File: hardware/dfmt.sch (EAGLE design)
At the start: 16 parts, among them X1 MINI-USB-32005-201

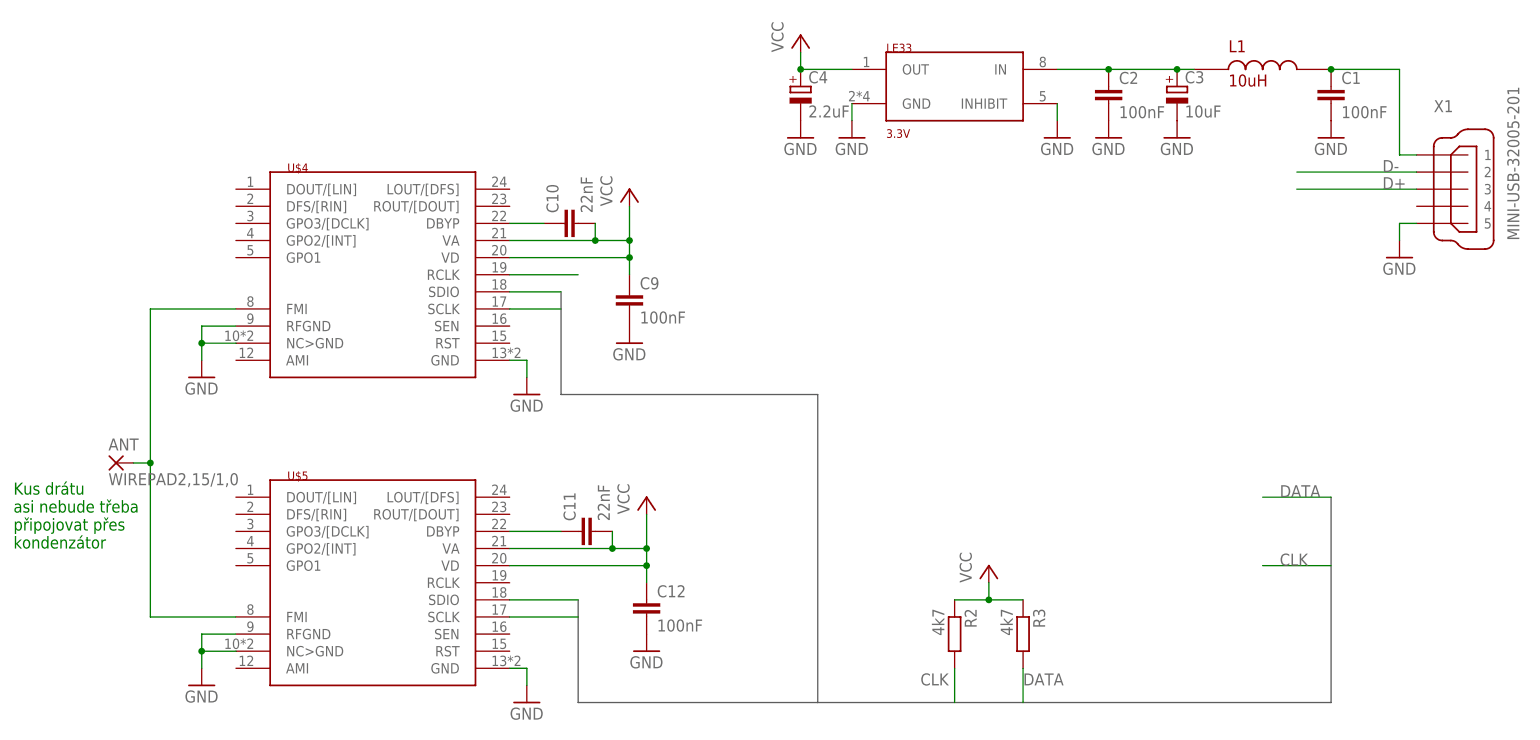
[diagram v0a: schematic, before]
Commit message: working version
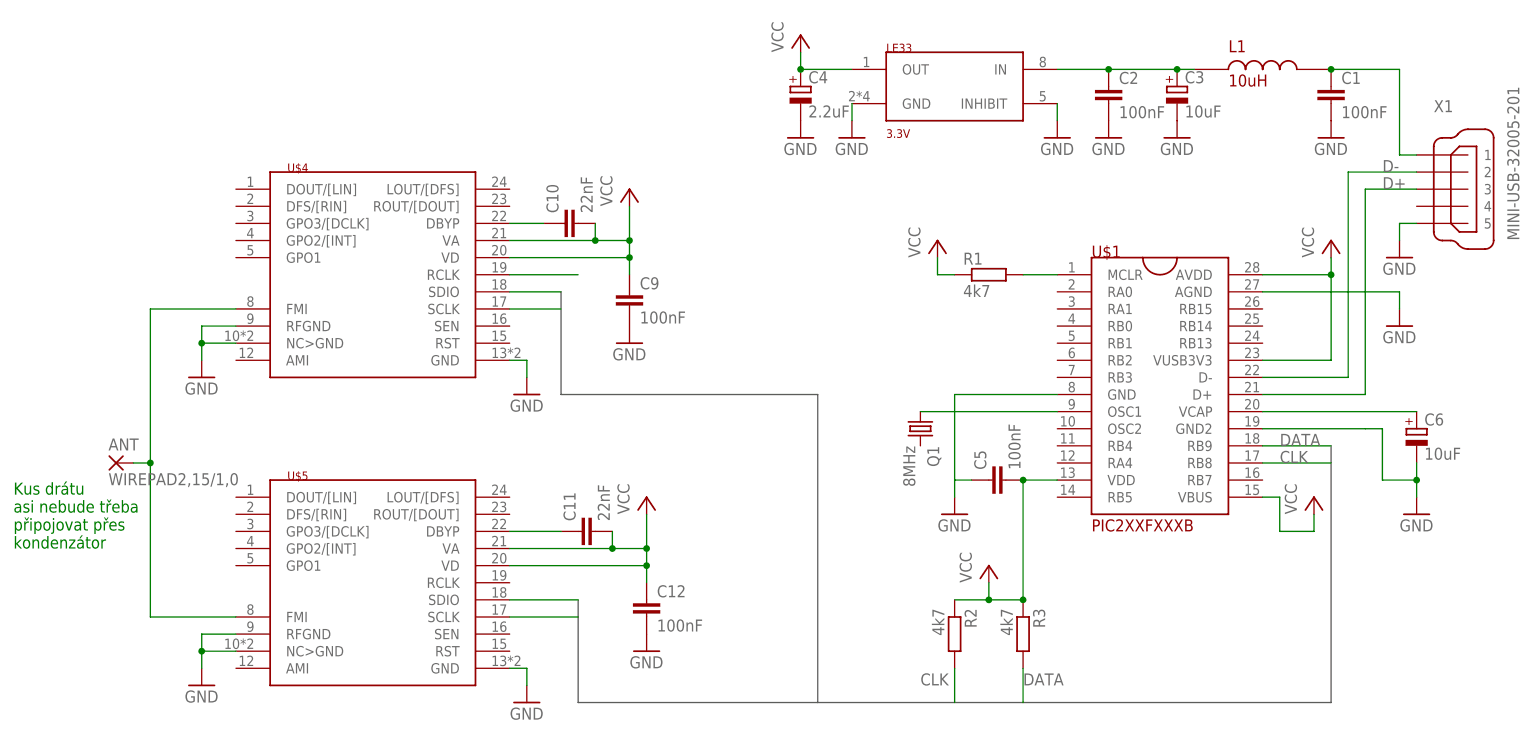
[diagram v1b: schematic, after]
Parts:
- added C5: 100nF, resistor:C-EUC1206
- added C6: 10uF, resistor:CPOL-EUSMCB
- added Q1: 8MHz, crystal:CSM-7X-DU
- added R1: 4k7, resistor:R-EU_R1206
- added U$1: PIC2XXFXXXB, dfmt:PIC2XXFXXXB
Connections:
- new net N$10: U$1.GND2
- new net N$11: Q1.1, U$1.OSC1
- new net N$5: R1.2, U$1.MCLR
- new net N$7: C6.+, U$1.VCAP
- net CLK: now also U$1.RB8
- net D+: now also U$1.D+
- net D-: now also U$1.D-
- net DATA: now also U$1.RB9
- net GND: now also C5.1, C6.-, U$1.AGND, U$1.GND
- net VCC: now also C5.2, R1.1, U$1.AVDD, U$1.VBUS, U$1.VDD, U$1.VUSB3V3
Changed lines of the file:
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@@
 <part name="X1" library="con-cypressindustries" deviceset="MINI-USB-" device="32005-201"/>
 <part name="GND7" library="supply1" deviceset="GND" device=""/>
+<part name="U$1" library="dfmt" deviceset="PIC2XXFXXXB" device=""/>
+<part name="GND8" library="supply1" deviceset="GND" device=""/>
+<part name="GND9" library="supply1" deviceset="GND" device=""/>
+<part name="P+2" library="supply1" deviceset="VCC" device=""/>
+<part name="R1" library="resistor" deviceset="R-EU_" device="R1206" value="4k7"/>
+<part name="P+6" library="supply1" deviceset="VCC" device=""/>
+<part name="C5" library="resistor" deviceset="C-EU" device="C1206" value="100nF"/>
+<part name="C6" library="resistor" deviceset="CPOL-EU" device="SMCB" value="10uF"/>
+<part name="GND16" library="supply1" deviceset="GND" device=""/>
+<part name="P+7" library="supply1" deviceset="VCC" device=""/>
+<part name="Q1" library="crystal" deviceset="CSM-7X-DU" device="" value="8MHz"/>
 </parts>
 <sheets>
@@
 <instance part="X1" gate="G$1" x="58.42" y="50.8"/>
 <instance part="GND7" gate="1" x="50.8" y="40.64"/>
+<instance part="U$1" gate="G$1" x="15.24" y="22.86"/>
+<instance part="GND8" gate="1" x="53.34" y="2.54"/>
+<instance part="GND9" gate="1" x="-15.24" y="2.54"/>
+<instance part="P+2" gate="VCC" x="40.64" y="43.18"/>
+<instance part="R1" gate="G$1" x="-10.16" y="38.1"/>
+<instance part="P+6" gate="VCC" x="-17.78" y="43.18"/>
+<instance part="C5" gate="G$1" x="-10.16" y="7.62" rot="R90"/>
+<instance part="C6" gate="G$1" x="53.34" y="15.24"/>
+<instance part="GND16" gate="1" x="50.8" y="30.48"/>
+<instance part="P+7" gate="VCC" x="38.1" y="5.08"/>
+<instance part="Q1" gate="P" x="-20.32" y="15.24" rot="R270"/>
 </instances>
 <busses>
 <bus name="DATA,CLK">
 <segment>
-<wire x1="40.64" y1="5.08" x2="40.64" y2="-25.4" width="0.762" layer="92"/>
+<wire x1="40.64" y1="12.7" x2="40.64" y2="-25.4" width="0.762" layer="92"/>
 <wire x1="40.64" y1="-25.4" x2="-35.56" y2="-25.4" width="0.762" layer="92"/>
 <wire x1="-35.56" y1="-25.4" x2="-71.12" y2="-25.4" width="0.762" layer="92"/>
@@
 <pinref part="X1" gate="G$1" pin="5"/>
 <wire x1="50.8" y1="45.72" x2="53.34" y2="45.72" width="0.1524" layer="91"/>
+</segment>
+<segment>
+<pinref part="C5" gate="G$1" pin="1"/>
+<pinref part="GND9" gate="1" pin="GND"/>
+<wire x1="-12.7" y1="7.62" x2="-15.24" y2="7.62" width="0.1524" layer="91"/>
+<wire x1="-15.24" y1="7.62" x2="-15.24" y2="5.08" width="0.1524" layer="91"/>
+<pinref part="U$1" gate="G$1" pin="GND"/>
+<wire x1="0" y1="20.32" x2="-15.24" y2="20.32" width="0.1524" layer="91"/>
+<wire x1="-15.24" y1="20.32" x2="-15.24" y2="7.62" width="0.1524" layer="91"/>
+</segment>
+<segment>
+<wire x1="48.26" y1="15.24" x2="45.72" y2="15.24" width="0.1524" layer="91"/>
+<pinref part="C6" gate="G$1" pin="-"/>
+<pinref part="GND8" gate="1" pin="GND"/>
+<wire x1="53.34" y1="5.08" x2="53.34" y2="7.62" width="0.1524" layer="91"/>
+<wire x1="53.34" y1="7.62" x2="53.34" y2="10.16" width="0.1524" layer="91"/>
+<junction x="53.34" y="7.62"/>
+<wire x1="53.34" y1="7.62" x2="48.26" y2="7.62" width="0.1524" layer="91"/>
+<wire x1="48.26" y1="7.62" x2="48.26" y2="15.24" width="0.1524" layer="91"/>
+</segment>
+<segment>
+<pinref part="U$1" gate="G$1" pin="AGND"/>
+<pinref part="GND16" gate="1" pin="GND"/>
+<wire x1="30.48" y1="35.56" x2="50.8" y2="35.56" width="0.1524" layer="91"/>
+<wire x1="50.8" y1="35.56" x2="50.8" y2="33.02" width="0.1524" layer="91"/>
 </segment>
 </net>
@@
 <wire x1="-10.16" y1="-10.16" x2="-10.16" y2="-7.62" width="0.1524" layer="91"/>
 <pinref part="R3" gate="G$1" pin="1"/>
+<junction x="-10.16" y="-10.16"/>
+<pinref part="U$1" gate="G$1" pin="VDD"/>
+<pinref part="C5" gate="G$1" pin="2"/>
 <wire x1="-5.08" y1="-10.16" x2="-10.16" y2="-10.16" width="0.1524" layer="91"/>
-<junction x="-10.16" y="-10.16"/>
+<wire x1="0" y1="7.62" x2="-5.08" y2="7.62" width="0.1524" layer="91"/>
+<wire x1="-5.08" y1="-10.16" x2="-5.08" y2="7.62" width="0.1524" layer="91"/>
+<junction x="-5.08" y="7.62"/>
+<junction x="-5.08" y="-10.16"/>
+</segment>
+<segment>
+<pinref part="U$1" gate="G$1" pin="VUSB3V3"/>
+<pinref part="P+2" gate="VCC" pin="VCC"/>
+<wire x1="30.48" y1="25.4" x2="40.64" y2="25.4" width="0.1524" layer="91"/>
+<wire x1="40.64" y1="25.4" x2="40.64" y2="38.1" width="0.1524" layer="91"/>
+<pinref part="U$1" gate="G$1" pin="AVDD"/>
+<wire x1="40.64" y1="38.1" x2="40.64" y2="40.64" width="0.1524" layer="91"/>
+<wire x1="30.48" y1="38.1" x2="40.64" y2="38.1" width="0.1524" layer="91"/>
+<junction x="40.64" y="38.1"/>
+</segment>
+<segment>
+<pinref part="R1" gate="G$1" pin="1"/>
+<pinref part="P+6" gate="VCC" pin="VCC"/>
+<wire x1="-15.24" y1="38.1" x2="-17.78" y2="38.1" width="0.1524" layer="91"/>
+<wire x1="-17.78" y1="38.1" x2="-17.78" y2="40.64" width="0.1524" layer="91"/>
+</segment>
+<segment>
+<pinref part="U$1" gate="G$1" pin="VBUS"/>
+<wire x1="30.48" y1="5.08" x2="33.02" y2="5.08" width="0.1524" layer="91"/>
+<wire x1="33.02" y1="5.08" x2="33.02" y2="0" width="0.1524" layer="91"/>
+<pinref part="P+7" gate="VCC" pin="VCC"/>
+<wire x1="33.02" y1="0" x2="38.1" y2="0" width="0.1524" layer="91"/>
+<wire x1="38.1" y1="0" x2="38.1" y2="2.54" width="0.1524" layer="91"/>
 </segment>
 </net>
@@
 <net name="DATA" class="0">
 <segment>
-<wire x1="40.64" y1="5.08" x2="30.48" y2="5.08" width="0.1524" layer="91"/>
-<label x="33.02" y="5.08" size="1.778" layer="95"/>
-</segment>
-<segment>
 <pinref part="U$5" gate="G$1" pin="SDIO"/>
 <wire x1="-71.12" y1="-10.16" x2="-81.28" y2="-10.16" width="0.1524" layer="91"/>
@@
 <label x="-5.08" y="-22.86" size="1.778" layer="95"/>
 </segment>
+<segment>
+<pinref part="U$1" gate="G$1" pin="RB9"/>
+<wire x1="40.64" y1="12.7" x2="30.48" y2="12.7" width="0.1524" layer="91"/>
+<label x="33.02" y="12.7" size="1.778" layer="95"/>
+</segment>
 </net>
 <net name="CLK" class="0">
-<segment>
-<wire x1="40.64" y1="-5.08" x2="30.48" y2="-5.08" width="0.1524" layer="91"/>
-<label x="33.02" y="-5.08" size="1.778" layer="95"/>
-</segment>
 <segment>
 <pinref part="U$5" gate="G$1" pin="SCLK"/>
@@
 <wire x1="-15.24" y1="-25.4" x2="-15.24" y2="-20.32" width="0.1524" layer="91"/>
 <label x="-20.32" y="-22.86" size="1.778" layer="95"/>
+</segment>
+<segment>
+<pinref part="U$1" gate="G$1" pin="RB8"/>
+<wire x1="40.64" y1="10.16" x2="30.48" y2="10.16" width="0.1524" layer="91"/>
+<label x="33.02" y="10.16" size="1.778" layer="95"/>
 </segment>
 </net>
@@
 <segment>
 <pinref part="X1" gate="G$1" pin="2"/>
-<wire x1="53.34" y1="53.34" x2="35.56" y2="53.34" width="0.1524" layer="91"/>
+<wire x1="53.34" y1="53.34" x2="43.18" y2="53.34" width="0.1524" layer="91"/>
 <label x="48.26" y="53.34" size="1.778" layer="95"/>
+<pinref part="U$1" gate="G$1" pin="D-"/>
+<wire x1="30.48" y1="22.86" x2="43.18" y2="22.86" width="0.1524" layer="91"/>
+<wire x1="43.18" y1="22.86" x2="43.18" y2="53.34" width="0.1524" layer="91"/>
 </segment>
 </net>
@@
 <segment>
 <pinref part="X1" gate="G$1" pin="3"/>
-<wire x1="53.34" y1="50.8" x2="35.56" y2="50.8" width="0.1524" layer="91"/>
+<wire x1="53.34" y1="50.8" x2="45.72" y2="50.8" width="0.1524" layer="91"/>
 <label x="48.26" y="50.8" size="1.778" layer="95"/>
-</segment>
-</net>
+<pinref part="U$1" gate="G$1" pin="D+"/>
+<wire x1="30.48" y1="20.32" x2="45.72" y2="20.32" width="0.1524" layer="91"/>
+<wire x1="45.72" y1="20.32" x2="45.72" y2="50.8" width="0.1524" layer="91"/>
+</segment>
+</net>
+<net name="N$5" class="0">
+<segment>
+<pinref part="U$1" gate="G$1" pin="MCLR"/>
+<pinref part="R1" gate="G$1" pin="2"/>
+<wire x1="0" y1="38.1" x2="-5.08" y2="38.1" width="0.1524" layer="91"/>
+</segment>
+</net>
+<net name="N$7" class="0">
+<segment>
+<pinref part="U$1" gate="G$1" pin="VCAP"/>
+<pinref part="C6" gate="G$1" pin="+"/>
+<wire x1="30.48" y1="17.78" x2="53.34" y2="17.78" width="0.1524" layer="91"/>
+</segment>
+</net>
+<net name="N$10" class="0">
+<segment>
+<pinref part="U$1" gate="G$1" pin="GND2"/>
+<wire x1="30.48" y1="15.24" x2="45.72" y2="15.24" width="0.1524" layer="91"/>
+</segment>
+</net>
+<net name="N$11" class="0">
+<segment>
+<pinref part="U$1" gate="G$1" pin="OSC1"/>
+<pinref part="Q1" gate="P" pin="1"/>
+<wire x1="0" y1="17.78" x2="-20.32" y2="17.78" width="0.1524" layer="91"/>
+</segment>
+</net>
